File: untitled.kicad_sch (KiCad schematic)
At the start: 17 parts, among them IC2 ADUM3221ARZ, IC3 ADUM3221ARZ, IC4 TLP188_TPL,E, IC5 TLP188_TPL,E, IC6 TLP188_TPL,E, IC7 TLP188_TPL,E, J5 Conn_01x10, J6 Conn_01x04, U4 K155NA1

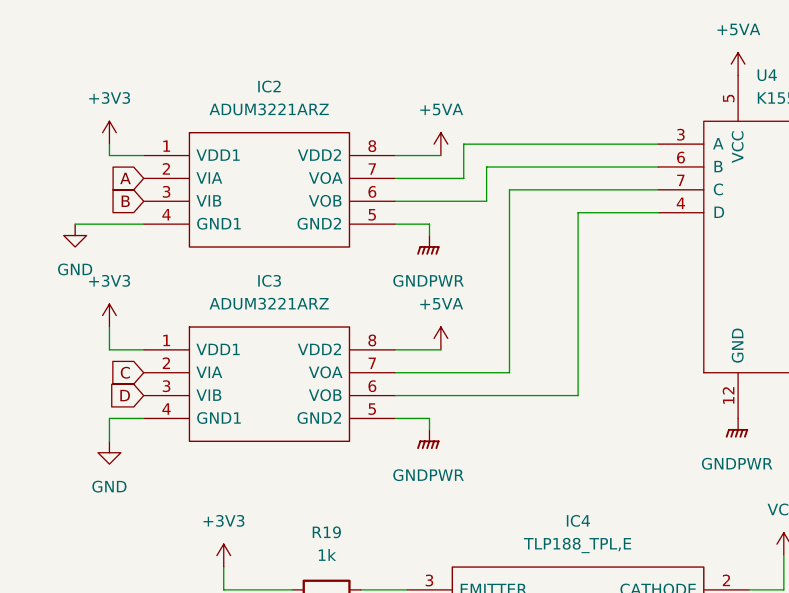
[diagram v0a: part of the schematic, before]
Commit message: upperside
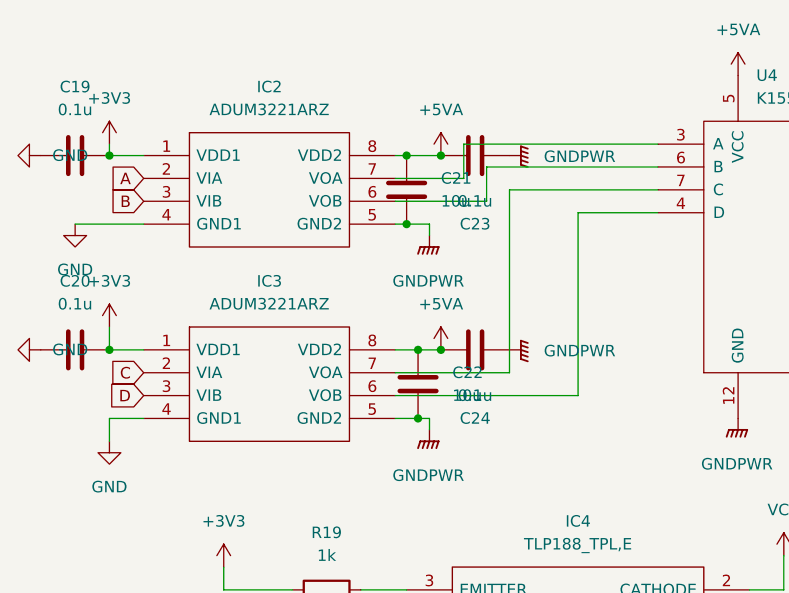
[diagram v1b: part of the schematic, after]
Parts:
- added C19, C20, C23, C24: 0.1u, Capacitor_SMD:C_0603_1608Metric_Pad1.08x0.95mm_HandSolder, symbol Device:C
- added C21, C22: 10u, Capacitor_SMD:C_0603_1608Metric_Pad1.08x0.95mm_HandSolder, symbol Device:C
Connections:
- net +3V3: now also C19.2, C20.2
- net +5VA: now also C21.2, C22.2, C23.2, C24.2
- net GND: now also C19.1, C20.1
- net GNDPWR: now also C21.1, C22.1, C23.1, C24.1
